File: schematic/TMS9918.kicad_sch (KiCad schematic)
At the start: 23 parts, among them J1 Bus, J2 Video out, J3 Power, J4 ext, Q1 2N4401, U1 TMS9918A, U2 HM62256BLP, U3 74HCT574, U4 74HCT574, U5 74HCT574, U6 74HCT04, Y1 10.738635MHz

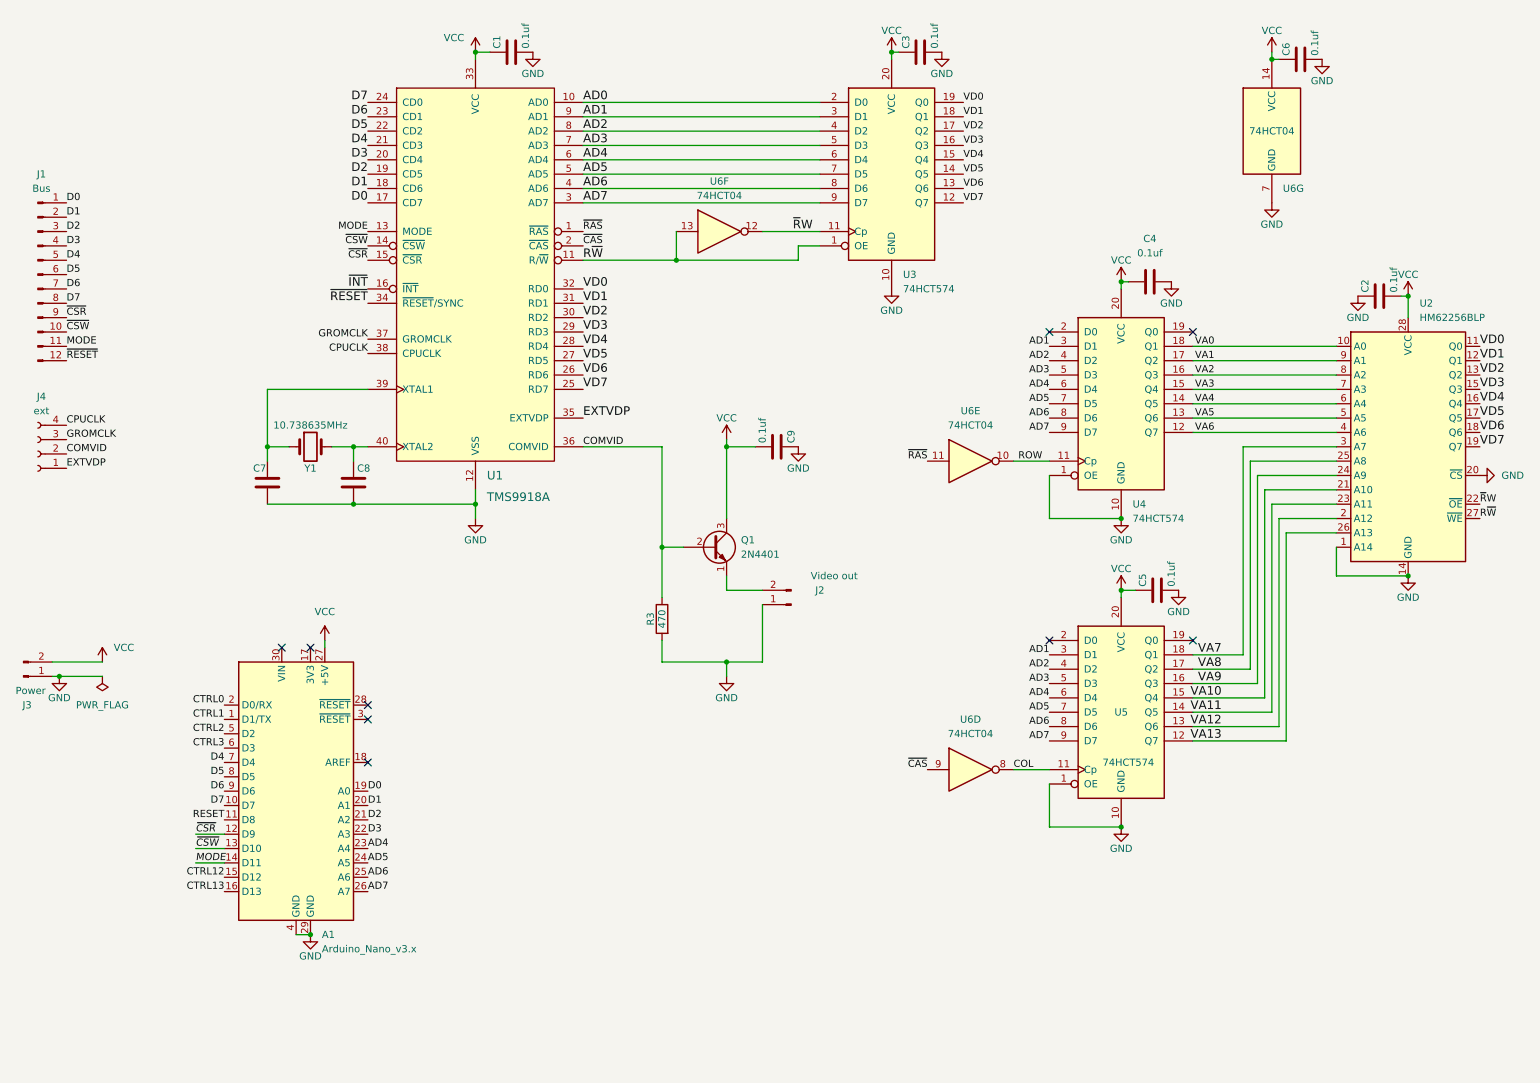
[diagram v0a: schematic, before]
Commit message: V1.1
Various improvements
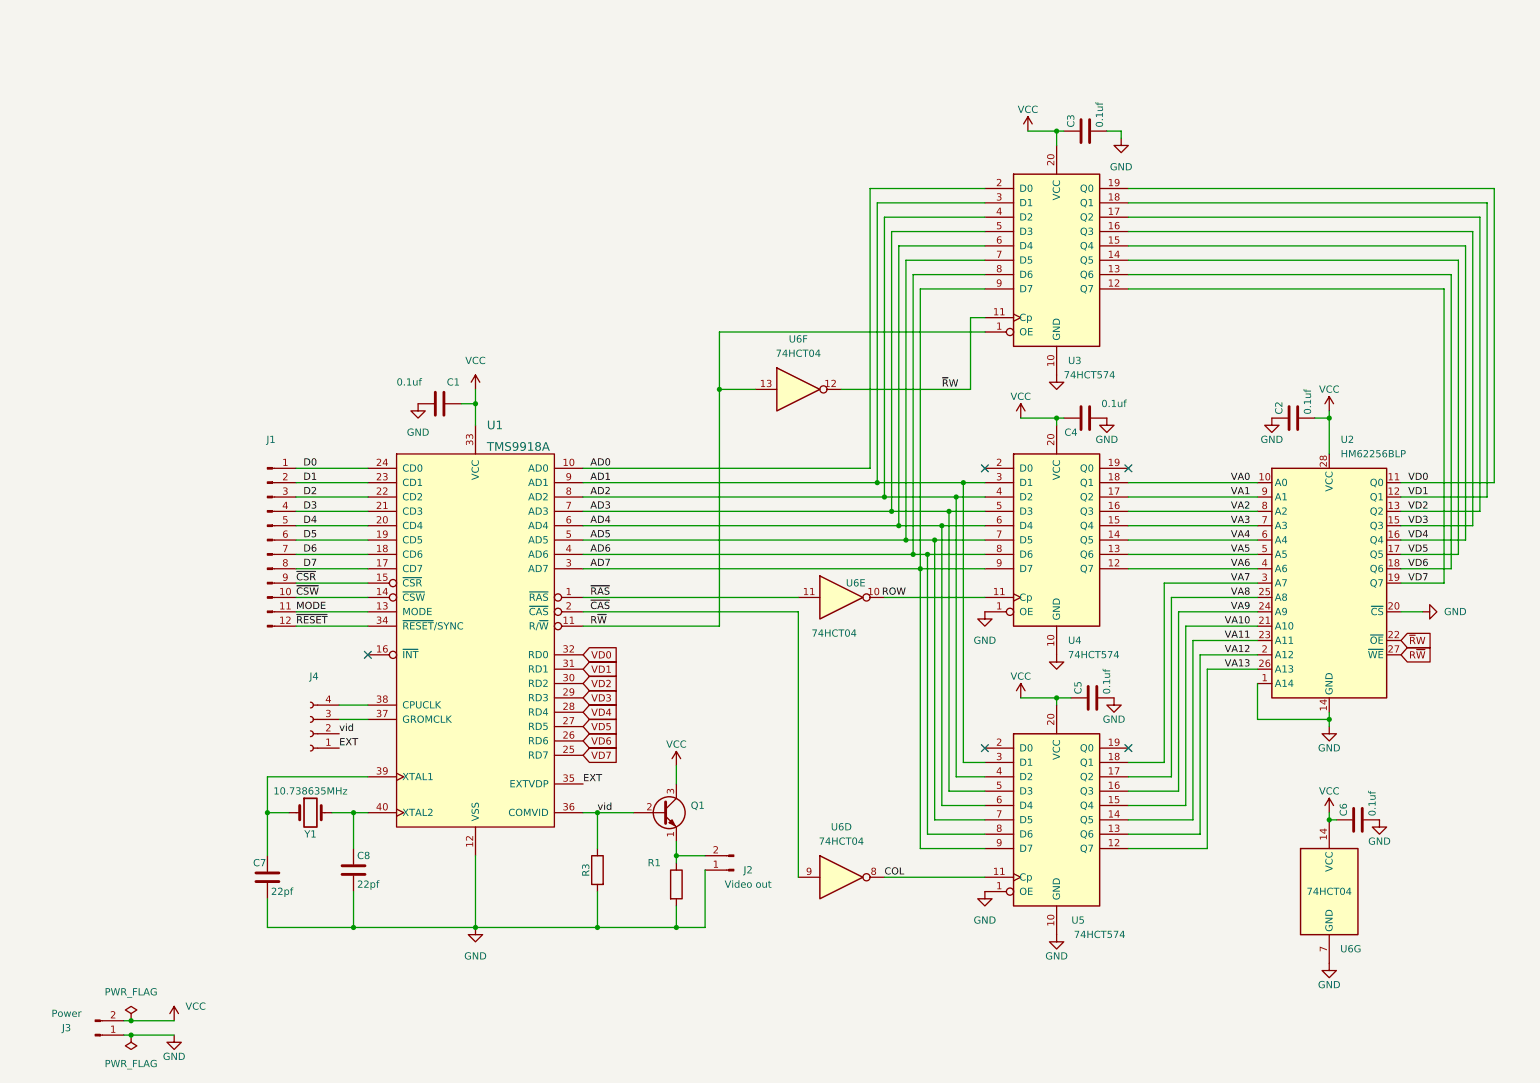
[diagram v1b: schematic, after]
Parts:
- removed A1: Arduino_Nano_v3.x, Module:Arduino_Nano, symbol MCU_Module:Arduino_Nano_v3.x
- removed C9: 0.1uf, Capacitor_THT:C_Disc_D3.0mm_W1.6mm_P2.50mm, symbol Device:C
- added R1: (no value), symbol Device:R
- C7, C8: value (none) -> 22pf
- J1: value Bus -> (none); footprint Connector_PinHeader_2.54mm:PinHeader_1x12_P2.54mm_Vertical -> (none)
- J4: value ext -> (none); footprint Connector_PinHeader_2.54mm:PinHeader_1x04_P2.54mm_Vertical -> (none)
- Q1: value 2N4401 -> (none); footprint Package_TO_SOT_THT:TO-92 -> (none)
- R3: value 470 -> (none)
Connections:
- net D0: now also U1.24 (CD0); no longer U1.17 (CD7)
- net D1: now also U1.23 (CD1); no longer U1.18 (CD6)
- net D2: now also U1.22 (CD2); no longer U1.19 (CD5)
- net D3: now also U1.21 (CD3); no longer U1.20 (CD4)
- net D4: now also U1.20 (CD4); no longer U1.21 (CD3)
- net D5: now also U1.19 (CD5); no longer U1.22 (CD2)
- net D6: now also U1.18 (CD6); no longer U1.23 (CD1)
- net D7: now also U1.17 (CD7); no longer U1.24 (CD0)
- net GND: now also R1.2
- net at J2.2 (Pin_2), Q1.1 (E): now also R1.1
- net COMVID renamed vid
- net CPUCLK: no longer names the net of J4.4 (Pin_4), U1.38 (CPUCLK)
- net EXTVDP renamed EXT
- net GROMCLK: no longer names the net of J4.3 (Pin_3), U1.37 (GROMCLK)
- net ~{INT}: no longer names the net of U1.16 (~{INT})
- no-connect marks 9 -> 5
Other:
- moved on the sheet: C2, C3, C4, C5, C6, U2, U3, U4, U5, U6D, U6E, U6F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
